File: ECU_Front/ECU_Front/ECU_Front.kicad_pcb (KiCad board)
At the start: 2 copper layers, 105 x 58 mm, 18 parts, among them J1 Conn_01x04_Pin, J2 Conn_01x04_Pin, U1 step-down (buck), U3 ESP32-DevKitC

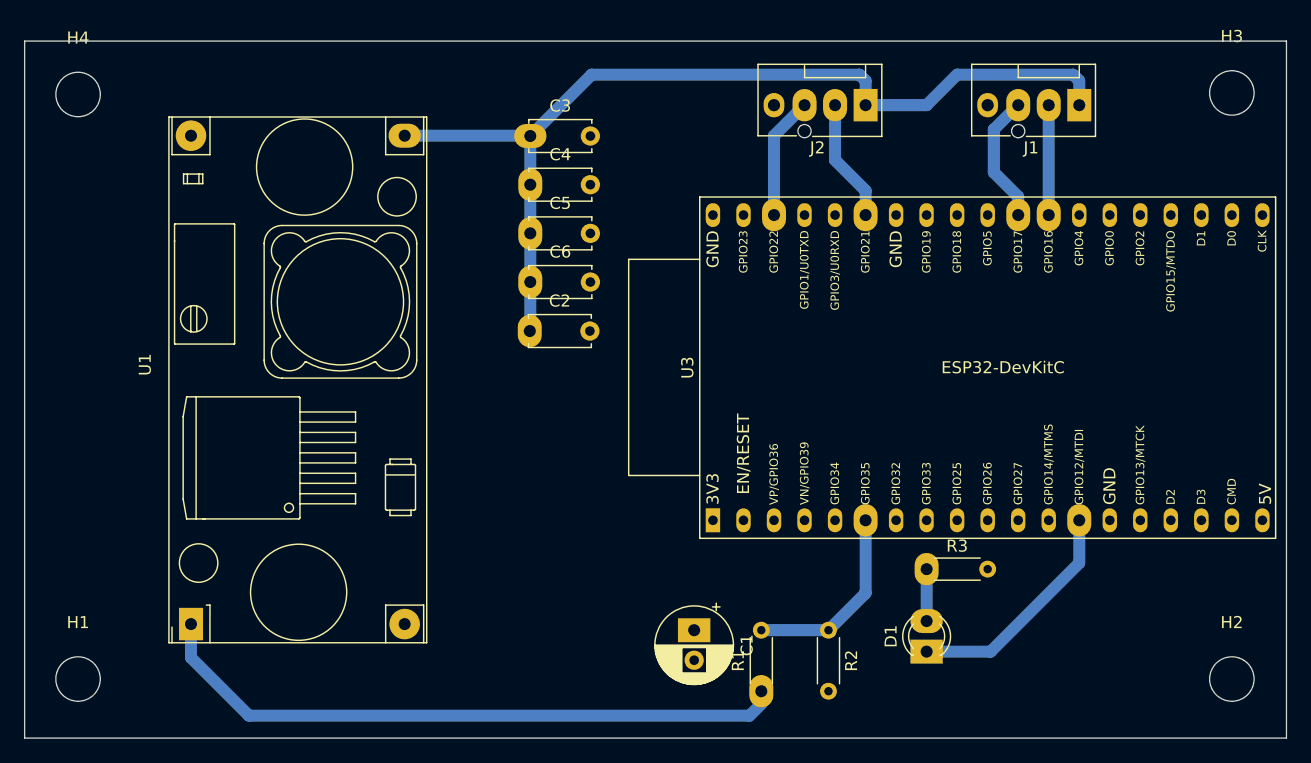
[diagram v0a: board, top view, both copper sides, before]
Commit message: ECU_Front, definitive edition
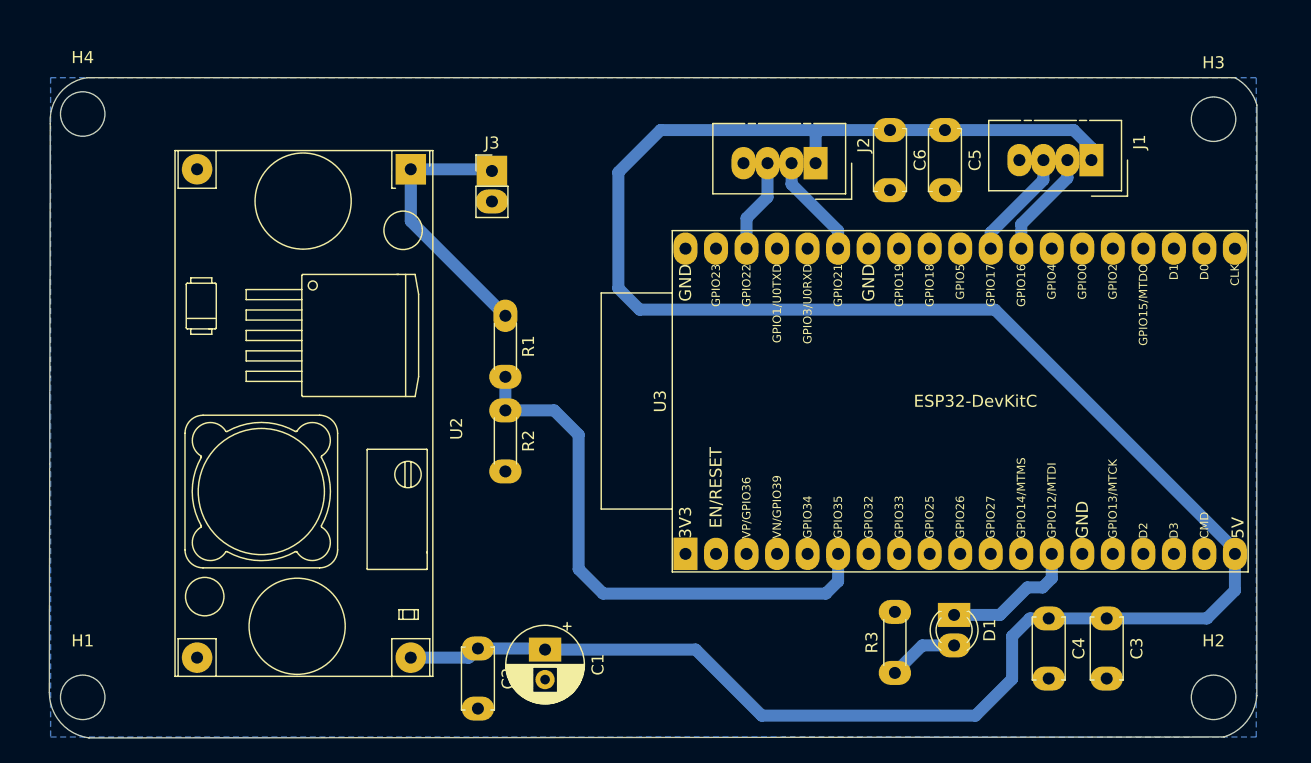
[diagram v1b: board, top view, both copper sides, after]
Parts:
- removed U1: step-down (buck), StepDown:StepDown_LM2596
- added J3: Conn_01x02_Pin, Connector_PinHeader_2.54mm:PinHeader_1x02_P2.54mm_Vertical, F.Cu at (146.2, 93.4)
- added U2: YAAJ_DCDC_StepDown_LM2596, StepDown:StepDown_LM2596, F.Cu at (139.4, 93.2)
- J1, J2: footprint Connector:FanPinHeader_1x04_P2.54mm_Vertical -> Connector:NS-Tech_Grove_1x04_P2mm_Vertical
- moved C3 62.5 mm to (197.4, 130.6), turned to -90 degrees
- moved C4 56.2 mm to (192.5, 130.6), turned to -90 degrees
- moved R1 37.8 mm to (147.3, 105.4), turned to -90 degrees
- moved C5 35.6 mm to (183.9, 90.0), turned to -90 degrees
- moved R2 32.5 mm to (147.3, 113.3)
- moved C6 32.5 mm to (179.3, 90.0), turned to -90 degrees
- moved C2 26.8 mm to (145.0, 133.1), turned to -90 degrees
- moved C1 12.5 mm to (150.6, 133.2)
- moved R3 9.03 mm to (179.7, 135.1), turned to 90 degrees
- moved J2 6.37 mm to (173.1, 92.7), turned to -90 degrees
- moved J1 4.68 mm to (196.1, 92.5), turned to -90 degrees
- moved D1 3.81 mm to (184.7, 130.3), turned to -90 degrees
- moved U3 3.61 mm to (162.3, 125.2)
- moved H3 2.66 mm to (206.2, 89.1)
- moved H2 2.16 mm to (206.2, 137.2)
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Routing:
- net +5V: track 80.0 -> 196.3 mm
- net +12V: track 53.9 -> 22.3 mm
- net VBAT-3V: track 16.0 -> 46.4 mm
- net LED_ALIVE: track 19.3 -> 11.4 mm
- net SCL: track 10.2 -> 7.84 mm
- net TXD2: track 10.8 -> 9.18 mm
- net Net-(D1-A): track 4.32 -> 5.87 mm
- net SDA: track 10.2 -> 8.72 mm
- added copper zone on B.Cu, net GND
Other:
- board size 105 x 58 mm -> 100.5 x 54.9 mm
